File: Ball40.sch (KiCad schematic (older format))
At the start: 82 parts, among them J1 Conn_01x08_Male, J2 USB_C_Receptacle_USB2.0, SW1 SW_Push, U1 SRV05-4, U2 ATmega32U4-AU, Y1 16MHz

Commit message: placed components in the PCB file
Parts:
- J1: footprint Connector_PinHeader_2.54mm:PinHeader_1x08_P2.54mm_Vertical -> Connector_JST:JST_SH_SM08B-SRSS-TB_1x08-1MP_P1.00mm_Horizontal
- J2: footprint Type-C:HRO-TYPE-C-31-M-12 -> Type-C:USB_C_GCT_USB4085
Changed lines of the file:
@@
 F 0 "J2" H 7557 3317 50  0000 C CNN
 F 1 "USB_C_Receptacle_USB2.0" H 7557 3226 50  0000 C CNN
-F 2 "Type-C:HRO-TYPE-C-31-M-12" H 7600 2450 50  0001 C CNN
+F 2 "Type-C:USB_C_GCT_USB4085" H 7600 2450 50  0001 C CNN
 F 3 "https://www.usb.org/sites/default/files/documents/usb_type-c.zip" H 7600 2450 50  0001 C CNN
 	1    7450 2450
@@
 F 0 "J1" V 6977 4278 50  0000 C CNN
 F 1 "Conn_01x08_Male" V 6886 4278 50  0000 C CNN
-F 2 "Connector_PinHeader_2.54mm:PinHeader_1x08_P2.54mm_Vertical" H 7050 4350 50  0001 C CNN
+F 2 "Connector_JST:JST_SH_SM08B-SRSS-TB_1x08-1MP_P1.00mm_Horizontal" H 7050 4350 50  0001 C CNN
 F 3 "~" H 7050 4350 50  0001 C CNN
 	1    7050 4350

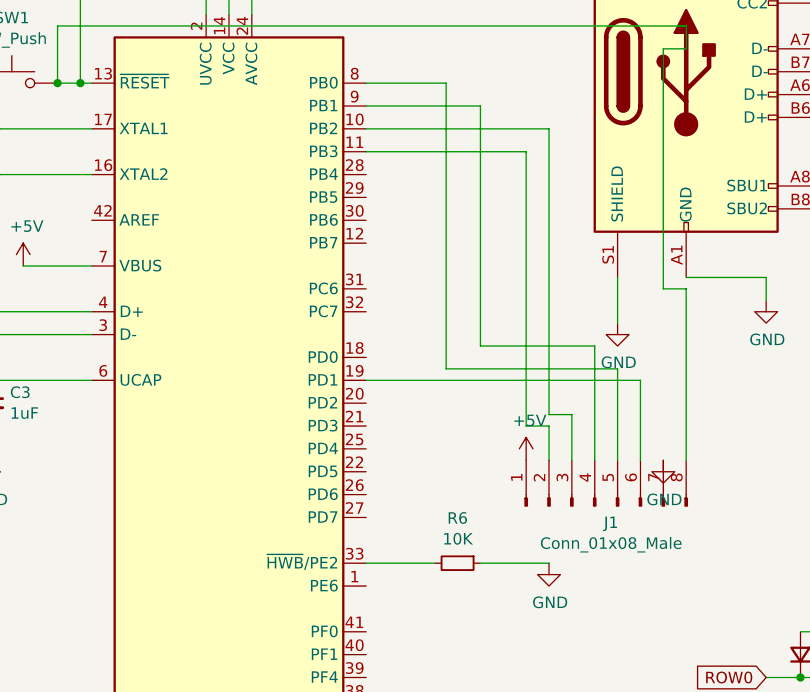
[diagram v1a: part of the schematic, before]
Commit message: generated gerbers
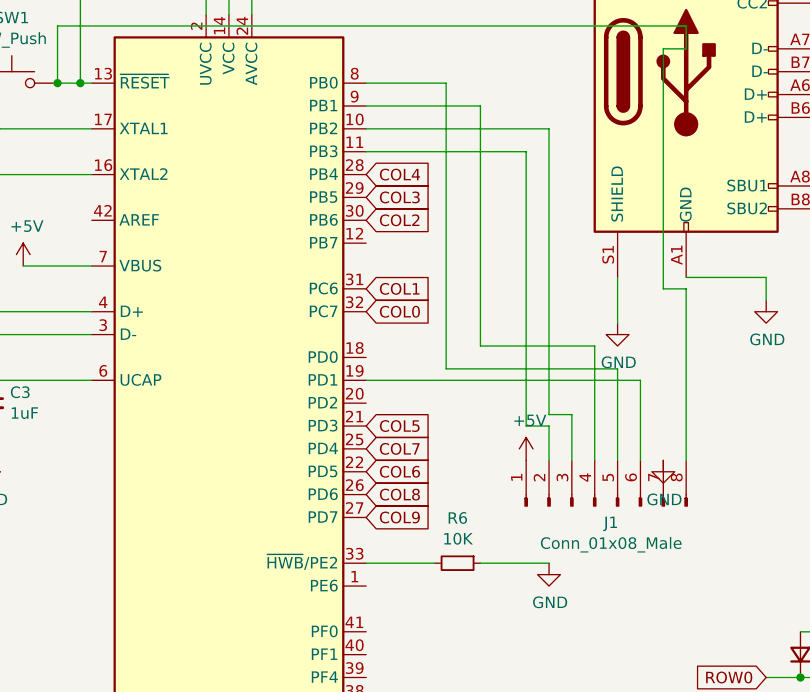
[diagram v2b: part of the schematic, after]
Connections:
- net COL0: now also U2.32 (PC7)
- net COL1: now also U2.31 (PC6)
- net COL2: now also U2.30 (PB6)
- net COL3: now also U2.29 (PB5)
- net COL4: now also U2.28 (PB4)
- net COL5: now also U2.21 (PD3)
- net COL6: now also U2.22 (PD5)
- net COL7: now also U2.25 (PD4)
- net COL8: now also U2.26 (PD6)
- net COL9: now also U2.27 (PD7)
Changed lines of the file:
@@
 	1    0    0    -1
 $EndComp
+Text GLabel 6050 4000 2    50   Input ~ 0
+COL5
+Text GLabel 6050 4200 2    50   Input ~ 0
+COL6
+Text GLabel 6050 4100 2    50   Input ~ 0
+COL7
+Text GLabel 6050 4300 2    50   Input ~ 0
+COL8
+Text GLabel 6050 4400 2    50   Input ~ 0
+COL9
+Text GLabel 6050 2900 2    50   Input ~ 0
+COL4
+Text GLabel 6050 3000 2    50   Input ~ 0
+COL3
+Text GLabel 6050 3100 2    50   Input ~ 0
+COL2
+Text GLabel 6050 3400 2    50   Input ~ 0
+COL1
+Text GLabel 6050 3500 2    50   Input ~ 0
+COL0
 $EndSCHEMATC
